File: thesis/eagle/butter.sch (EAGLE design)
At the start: 4 parts

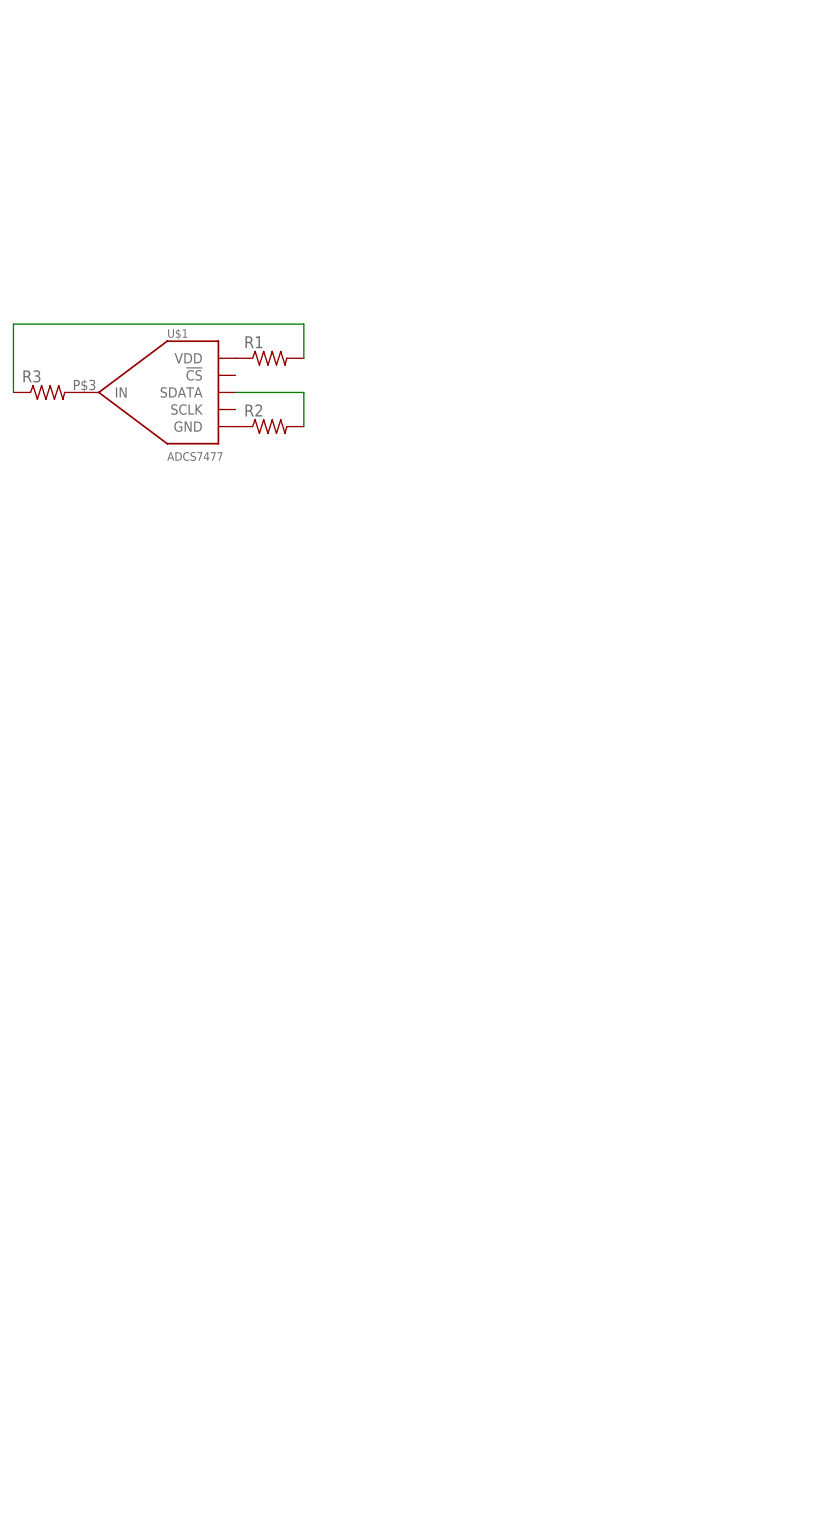
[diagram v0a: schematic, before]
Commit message: added eagle files for reals now
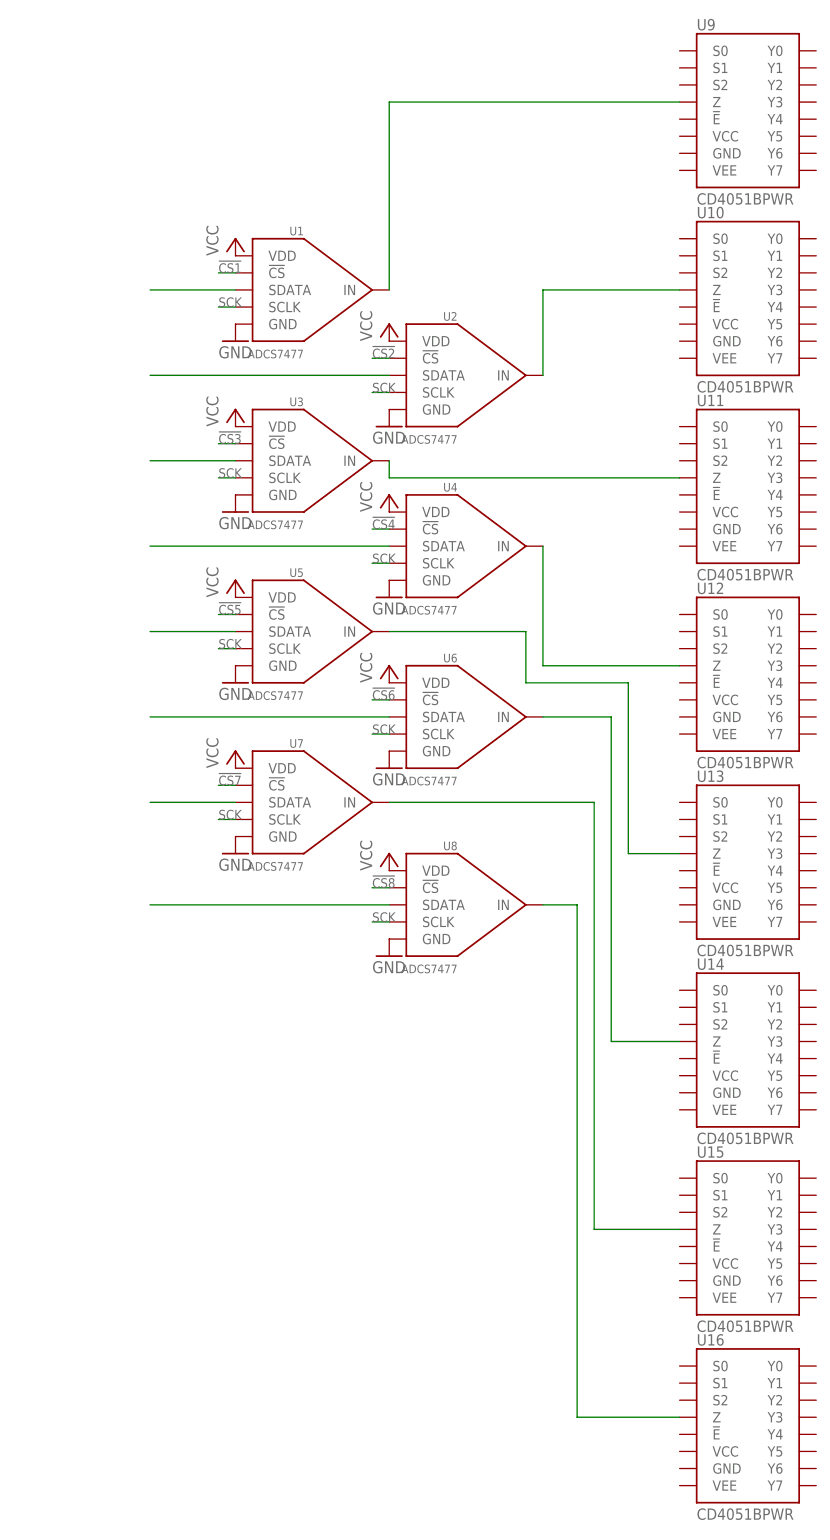
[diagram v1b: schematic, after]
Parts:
- removed R1, R2, R3: (no value), resistor:R-US_0414/5V
- removed U$1: ADCS7477, butter:ADCS7477
- added U1, U2, U3, U4, U5, U6, U7, U8: ADCS7477, butter:ADCS7477
- added U10, U11, U12, U13, U14, U15, U16, U9: CD4051BPWR, butter:CD4051BPWR
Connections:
- new net !CS1: U1.!CS
- new net !CS2: U2.!CS
- new net !CS3: U3.!CS
- new net !CS4: U4.!CS
- new net !CS5: U5.!CS
- new net !CS6: U6.!CS
- new net !CS7: U7.!CS
- new net !CS8: U8.!CS
- new net D1: U1.SDATA
- new net D2: U2.SDATA
- new net D3: U3.SDATA
- new net D4: U4.SDATA
- new net D5: U5.SDATA
- new net D6: U6.SDATA
- new net D7: U7.SDATA
- new net D8: U8.SDATA
- new net GND: U1.GND, U2.GND, U3.GND, U4.GND, U5.GND, U6.GND, U7.GND, U8.GND
- new net N$6: U14.Z, U6.IN
- new net N$7: U15.Z, U7.IN
- new net N$8: U16.Z, U8.IN
- new net SCK: U1.SCLK, U2.SCLK, U3.SCLK, U4.SCLK, U5.SCLK, U6.SCLK, U7.SCLK, U8.SCLK
- new net VCC: U1.VDD, U2.VDD, U3.VDD, U4.VDD, U5.VDD, U6.VDD, U7.VDD, U8.VDD
- net N$1: now also U1.IN, U9.Z; no longer R1.1, U$1.VDD
- net N$2: now also U10.Z, U2.IN; no longer R2.1, U$1.GND
- net N$3: now also U11.Z, U3.IN; no longer R3.2, U$1.IN
- net N$4: now also U12.Z, U4.IN; no longer R1.2, R3.1
- net N$5: now also U13.Z, U5.IN; no longer R2.2, U$1.SDATA
